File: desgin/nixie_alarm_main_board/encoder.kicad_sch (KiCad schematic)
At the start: 7 parts

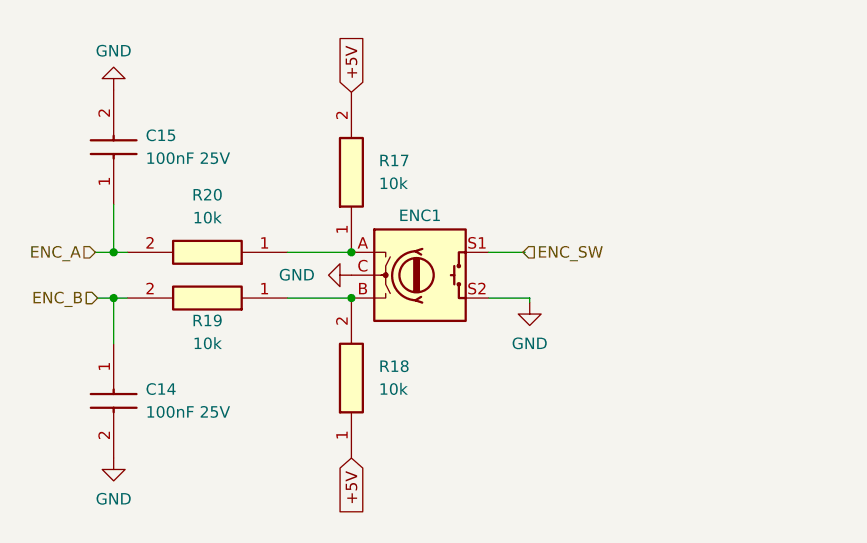
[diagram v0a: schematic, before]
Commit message: filter caps
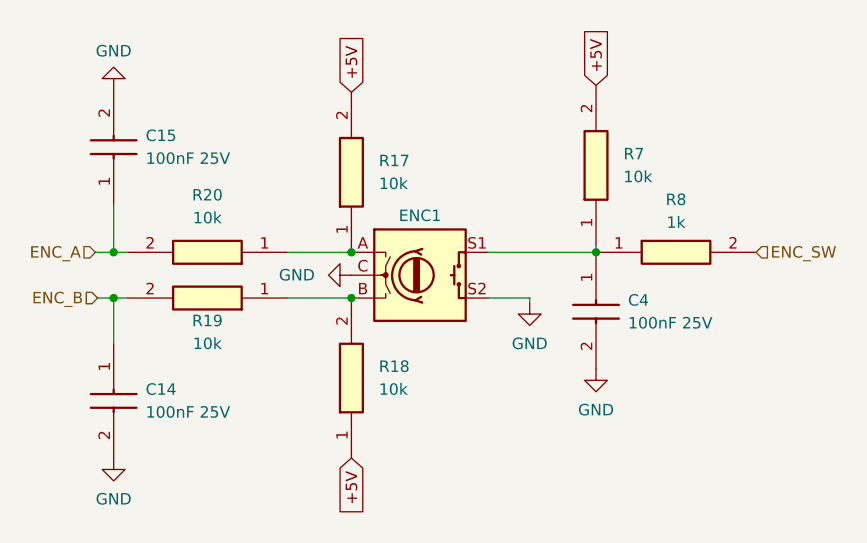
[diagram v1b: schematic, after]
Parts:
- added C4: 100nF 25V, GRM033D70J224ME01D, symbol SamacSys_Parts:GRM033R71E101KA01J
- added R7: 10k, ERJUP6, symbol SamacSys_Parts:ERJ-UP6D5101V
- added R8: 1k, ERJUP6, symbol SamacSys_Parts:ERJ-UP6D5101V
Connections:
- net +5V: now also R7.2
- net ENC_SW: now also R8.2; no longer ENC1.S1
- net GND: now also C4.2
- new net: C4.1, ENC1.S1, R7.1, R8.1
